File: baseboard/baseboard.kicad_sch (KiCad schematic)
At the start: 21 parts, among them IC1 ATA6561-GAQW-N, IC2 NJM2845DL1-33-TE1, J10 Conn_01x01_Pin, J9 A295-CTRPB-1, U1 PY32E407V1xT_START

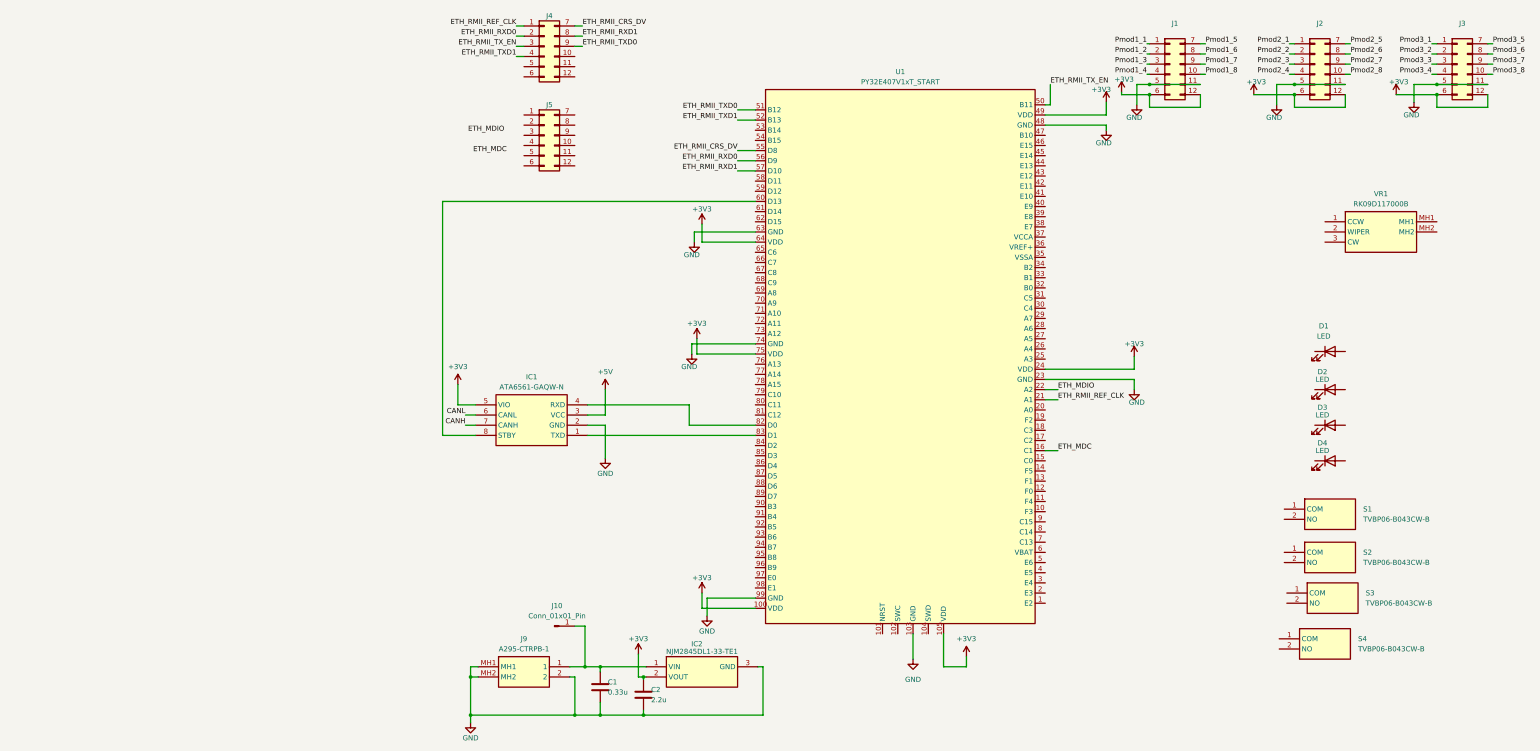
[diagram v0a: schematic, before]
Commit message: schematics can
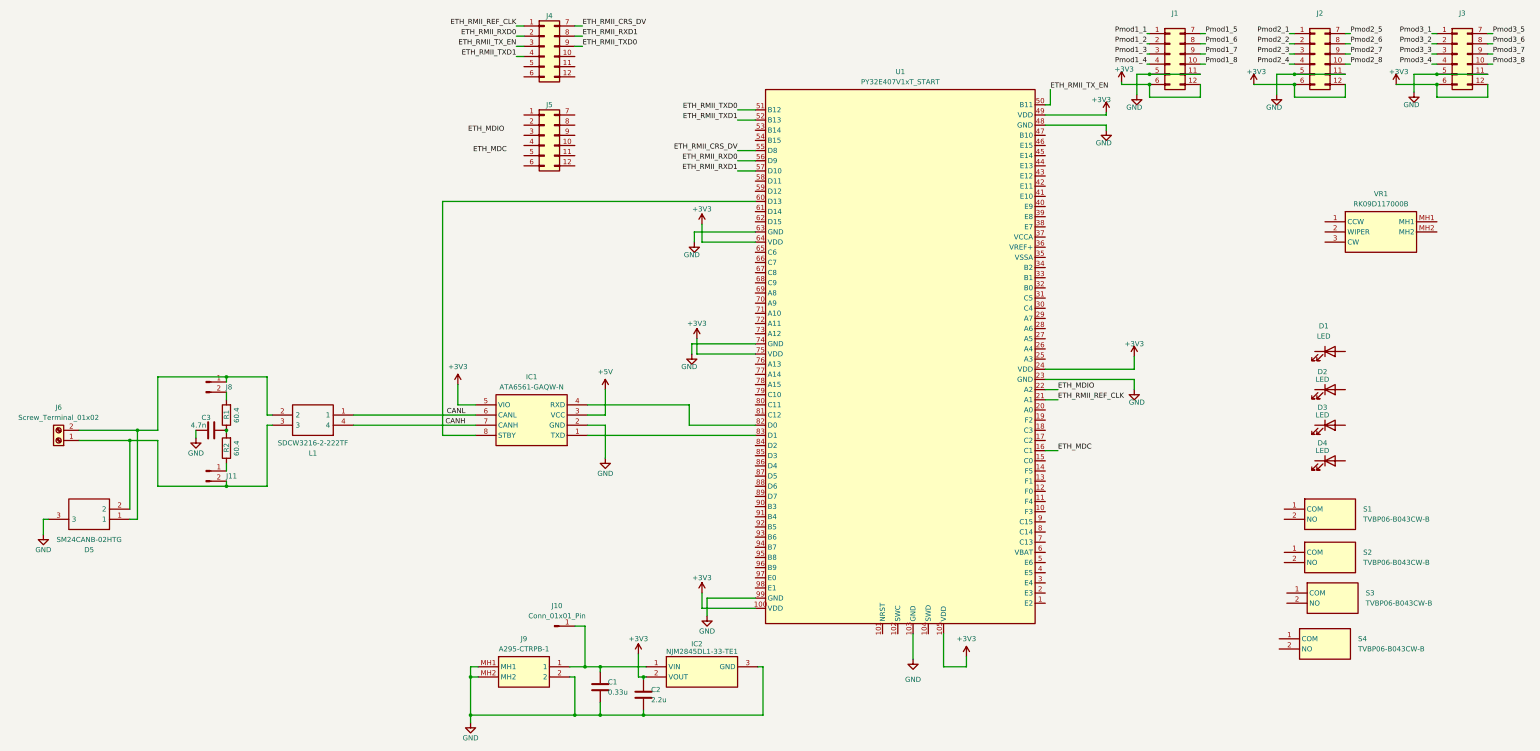
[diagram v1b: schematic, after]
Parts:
- added C3: 4.7n, Capacitor_SMD:C_0603_1608Metric_Pad1.08x0.95mm_HandSolder, symbol Device:C
- added D5: SM24CANB-02HTG, samacsys:SM24CANB02HTG, symbol samacsys:SM24CANB-02HTG
- added J11, J8: Conn_01x02_Pin, Connector_PinHeader_2.54mm:PinHeader_1x02_P2.54mm_Vertical, symbol Connector:Conn_01x02_Pin
- added J6: Screw_Terminal_01x02, TerminalBlock_Phoenix:TerminalBlock_Phoenix_MKDS-1,5-2-5.08_1x02_P5.08mm_Horizontal, symbol Connector:Screw_Terminal_01x02
- added L1: SDCW3216-2-222TF, samacsys:SDCW32162222TF, symbol samacsys:SDCW3216-2-222TF
- added R1, R2: 60.4, Resistor_SMD:R_0603_1608Metric_Pad0.98x0.95mm_HandSolder, symbol Device:R
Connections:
- net CANH: now also L1.4
- net CANL: now also L1.1
- net GND: now also C3.2, D5.3
- new net: J11.1 (Pin_1), R2.1
- new net: D5.2, J11.2 (Pin_2), J6.1 (Pin_1), L1.3
- new net: D5.1, J6.2 (Pin_2), J8.1 (Pin_1), L1.2
- new net: C3.1, R1.1, R2.2
- new net: J8.2 (Pin_2), R1.2
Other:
- moved on the sheet: J1, J2, J3
